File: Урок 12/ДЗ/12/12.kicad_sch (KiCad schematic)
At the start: 12 parts

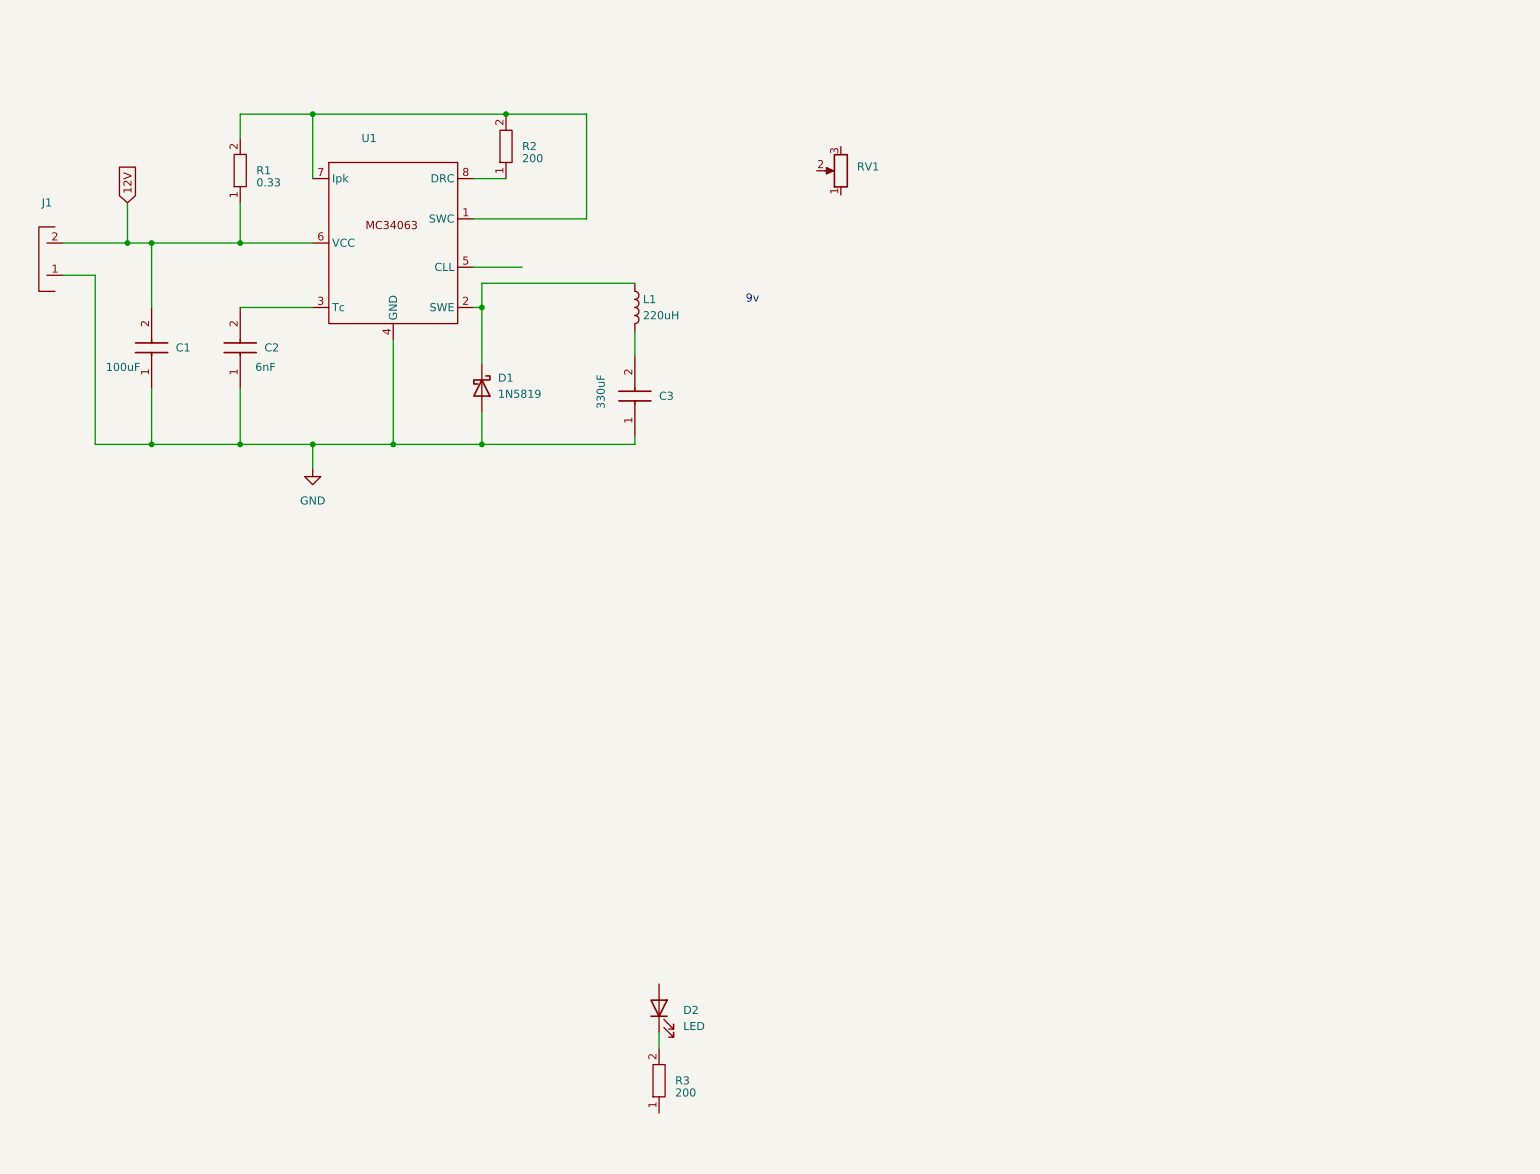
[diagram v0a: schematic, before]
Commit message: 12
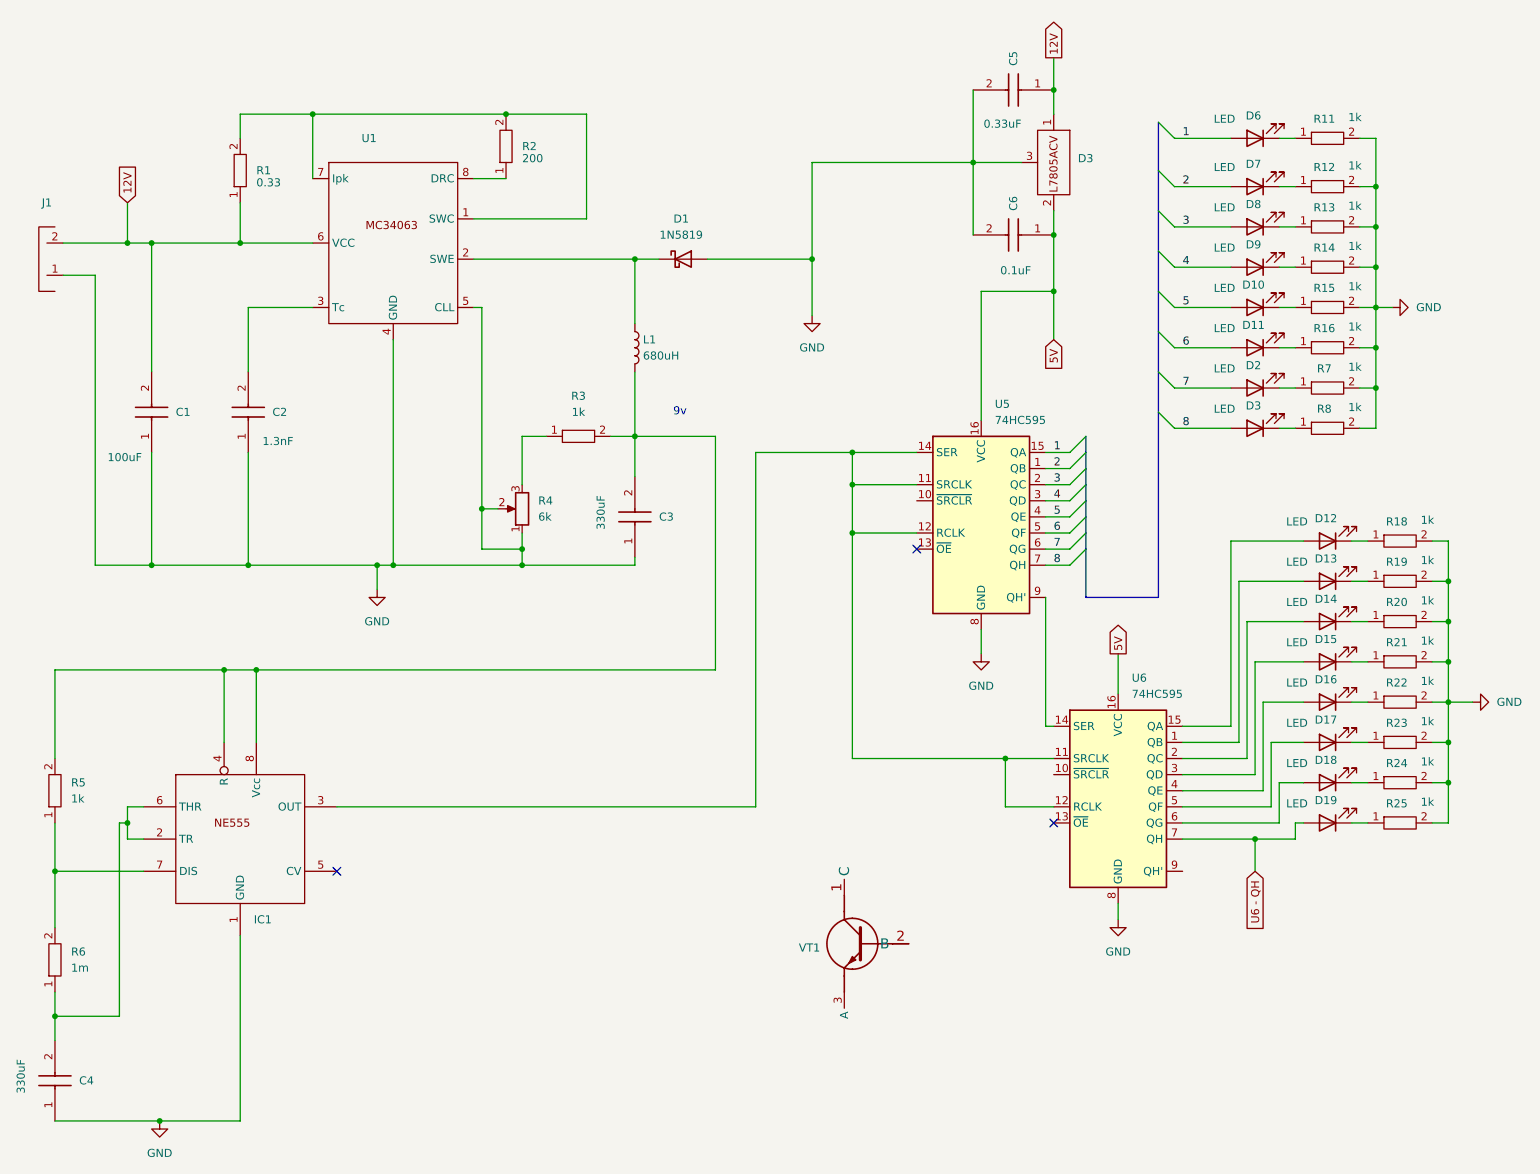
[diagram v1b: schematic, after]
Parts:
- removed RV1: ~, symbol My_Lib:R_Potentiometer
- added C4: 330uF, My_lib2:564R60GAD10, symbol My_Lib:C - 564R60GAD10
- added C5: 0.33uF, My_lib2:564R60GAD10, symbol My_Lib:C - 564R60GAD10
- added C6: 0.1uF, My_lib2:564R60GAD10, symbol My_Lib:C - 564R60GAD10
- added D10, D11, D12, D13, D14, D15, D16, D17, D18, D19, D3, D6, D7, D8, D9: LED, symbol My_Lib:LED
- added D3: ~, My_lib2:TO-220 - L7805ACV, symbol My_Lib:L7805ACV
- added IC1: ~, My_lib2:8-DIP, symbol My_Lib:NE555
- added R11, R12, R13, R14, R15, R16, R18, R19, R20, R21, R22, R23, R24, R25, R5, R7, R8: 1k, RESAD2700W60L1100D400, symbol My_Lib:R - CF100-3K3-J-TB-070-62
- added R4: 6k, symbol My_Lib:R_Potentiometer
- added R6: 1m, RESAD2700W60L1100D400, symbol My_Lib:R - CF100-3K3-J-TB-070-62
- added U5, U6: 74HC595, symbol 74xx:74HC595
- added VT1: ~, My_lib2:VT - BC32725PBFREE TO-92, symbol My_Lib:VT - КТ3102БМ
- C2: value 6nF -> 1.3nF
- L1: value 220uH -> 680uH
- R3: value 200 -> 1k
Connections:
- net 12V: now also C5.1, D3.1
- net GND: now also U1.5 (CLL), C4.1, C5.2, C6.2, D3.3 (GND), IC1.1 (GND), R11.2, R12.2, R13.2, R14.2, R15.2, R16.2, R18.2, R19.2, R20.2, R21.2, R22.2, R23.2, R24.2, R25.2, R4.1, R4.2, R7.2, R8.2, U5.8 (GND), U6.8 (GND)
- net at C3.2, L1.2: now also R3.2, IC1.4 (R), IC1.8 (Vcc), R5.2
- net at D2.1 (K): now also R7.1; no longer R3.2
- net 7: now reaches D2.2 (A)
- net 7: now also U5.6 (QG)
- net at R3.1: now also R4.3
- new net: C4.2, IC1.2 (TR), IC1.6 (THR), R6.1
- new net: D6.1 (K), R11.1
- new net: D7.1 (K), R12.1
- new net: D11.1 (K), R16.1
- new net: IC1.3 (OUT), U5.11 (SRCLK), U5.12 (RCLK), U5.14 (SER), U6.11 (SRCLK), U6.12 (RCLK)
- new net: U5.9 (QH'), U6.14 (SER)
- new net: D18.1 (K), R24.1
- new net: D18.2 (A), U6.6 (QG)
- new net: D3.1 (K), R8.1
- new net: D10.1 (K), R15.1
- new net: IC1.7 (DIS), R5.1, R6.2
- new net: D19.1 (K), R25.1
- new net: D14.1 (K), R20.1
- new net: D14.2 (A), U6.2 (QC)
- new net: D8.1 (K), R13.1
- new net: D9.1 (K), R14.1
- new net: D12.1 (K), R18.1
- new net: D12.2 (A), U6.15 (QA)
- new net: D13.2 (A), U6.1 (QB)
- new net: D15.2 (A), U6.3 (QD)
- new net: D16.2 (A), U6.4 (QE)
- new net: D17.2 (A), U6.5 (QF)
- new net: D16.1 (K), R22.1
- new net: D15.1 (K), R21.1
- new net: D17.1 (K), R23.1
- new net: D13.1 (K), R19.1
- new net 1: D6.2 (A), U5.15 (QA)
- new net 2: D7.2 (A), U5.1 (QB)
- new net 3: D8.2 (A), U5.2 (QC)
- new net 4: D9.2 (A), U5.3 (QD)
- new net 5: D10.2 (A), U5.4 (QE)
- new net 5V: C6.1, D3.2, U5.16 (VCC), U6.16 (VCC)
- new net 6: D11.2 (A), U5.5 (QF)
- new net 8: D3.2 (A), U5.7 (QH)
- new net U6 - QH: D19.2 (A), U6.7 (QH)
- no-connect marks 0 -> 3
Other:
- moved on the sheet: C1, C2, C3, D1, L1

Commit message: 12
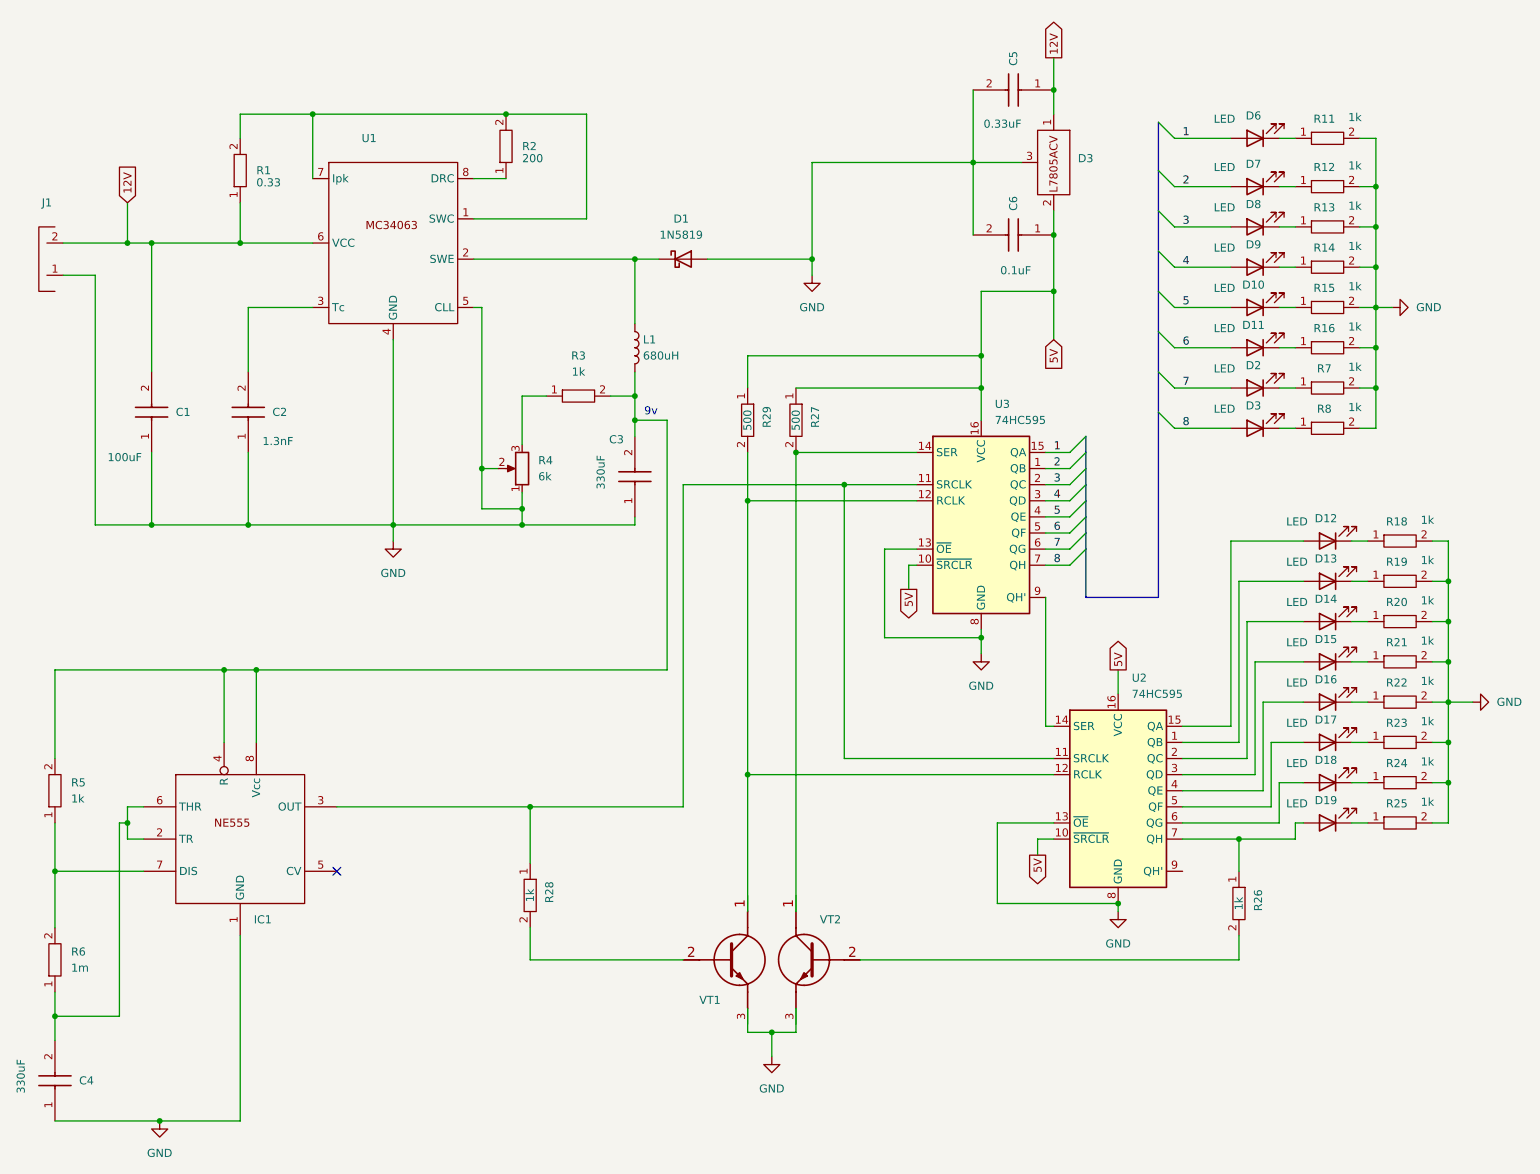
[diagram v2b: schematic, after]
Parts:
- removed U5, U6: 74HC595, symbol 74xx:74HC595
- added R26, R28: 1k, RESAD2700W60L1100D400, symbol My_Lib:R - CF100-3K3-J-TB-070-62
- added R27, R29: 500, RESAD2700W60L1100D400, symbol My_Lib:R - CF100-3K3-J-TB-070-62
- added U2, U3: 74HC595, symbol My_Lib:74HC595
- added VT1: ~, My_lib2:VT - BC32725PBFREE TO-92, symbol My_Lib:VT - КТ3102БМ
- renumbered VT1 to VT2
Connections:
- net 1: now also U3.15 (QA)
- net 2: now also U3.1 (QB)
- net 3: now also U3.2 (QC)
- net 4: now also U3.3 (QD)
- net 5: now also U3.4 (QE)
- net 5V: now also R27.1, R29.1, U2.10 (~{SRCLR}), U2.16 (VCC), U3.10 (~{SRCLR}), U3.16 (VCC)
- net 6: now also U3.5 (QF)
- net 7: now also U3.6 (QG)
- net 8: now also U3.7 (QH)
- net GND: now also VT2.3 (A), U2.13 (~{OE}), U2.8 (GND), U3.13 (~{OE}), U3.8 (GND), VT1.3 (A)
- net at IC1.3 (OUT): now also R28.1, U2.11 (SRCLK), U3.11 (SRCLK)
- net at D18.2 (A): now also U2.6 (QG)
- net at D14.2 (A): now also U2.2 (QC)
- net at D12.2 (A): now also U2.15 (QA)
- net at D13.2 (A): now also U2.1 (QB)
- net at D15.2 (A): now also U2.3 (QD)
- net at D16.2 (A): now also U2.4 (QE)
- net at D17.2 (A): now also U2.5 (QF)
- net at VT2.1 (C): now also R27.2, U3.14 (SER)
- net at VT2.2 (B): now also R26.2
- net U6 - QH: no longer names the net of D19.2 (A)
- net U6 - QH: now also R26.1, U2.7 (QH)
- new net: R29.2, U2.12 (RCLK), U3.12 (RCLK), VT1.1 (C)
- new net: U2.14 (SER), U3.9 (QH')
- new net: R28.2, VT1.2 (B)
- no-connect marks 3 -> 1
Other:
- moved on the sheet: C3, R3, R4
